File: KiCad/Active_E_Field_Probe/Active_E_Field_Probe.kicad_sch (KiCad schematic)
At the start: 11 parts

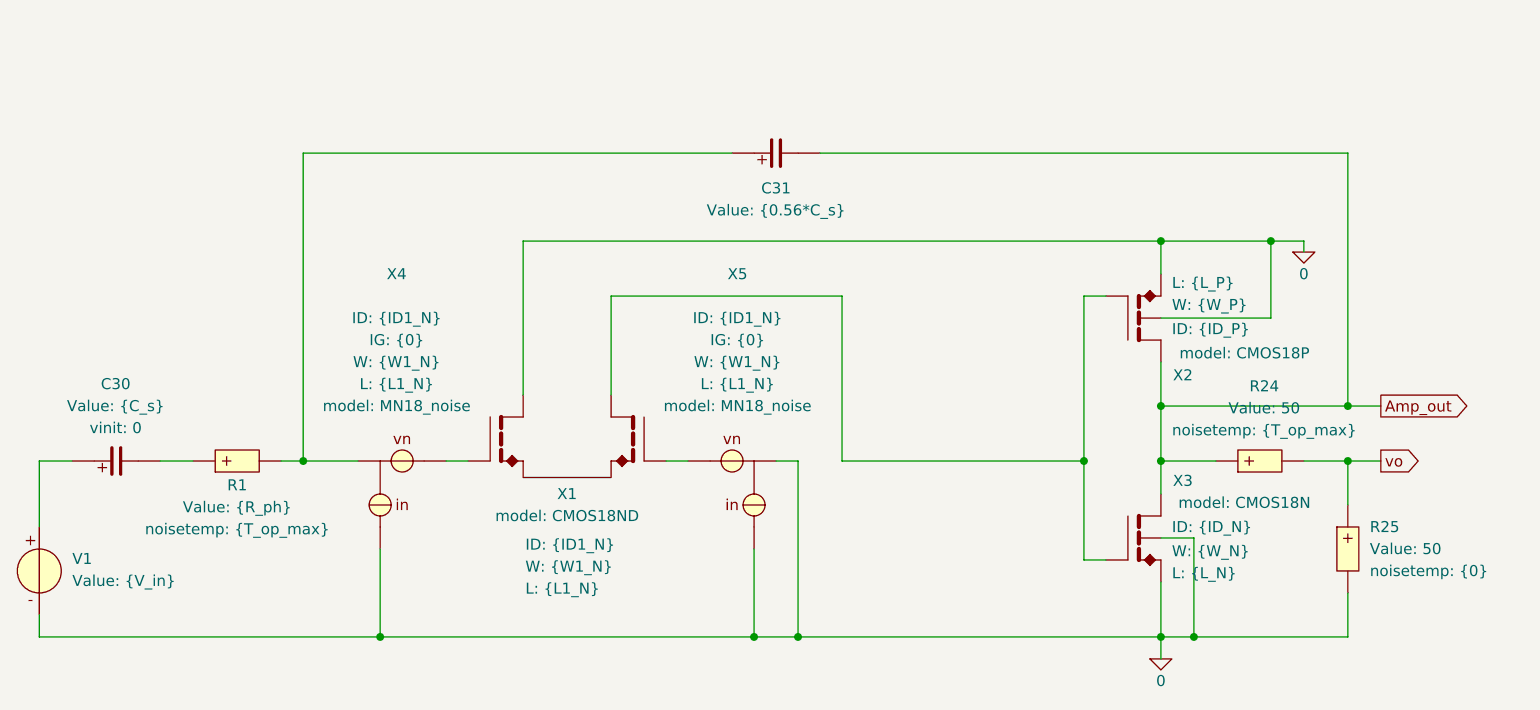
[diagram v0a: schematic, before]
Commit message: cascode
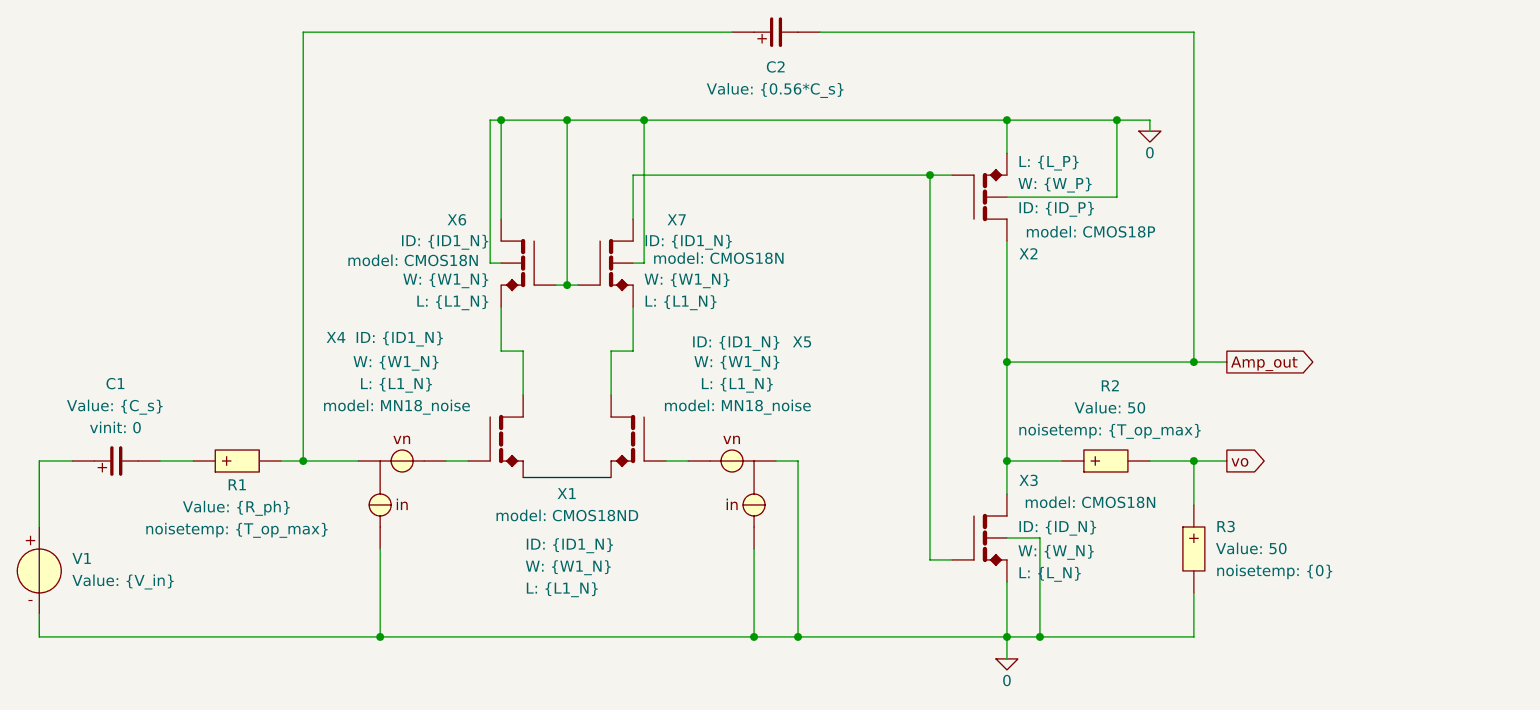
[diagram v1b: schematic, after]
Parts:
- added X6, X7: ~, symbol SLiCAP:XM
- renumbered C30 to C1, C31 to C2, R24 to R2, R25 to R3
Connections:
- net 0: now also X6.1 (D), X6.2 (G), X6.4 (B), X7.2 (G), X7.4 (B); no longer X1.1 (D1)
- net at X2.2 (G), X3.2 (G): now also X7.1 (D); no longer X1.2 (D2)
- new net: X1.2 (D2), X7.3 (S)
- new net: X1.1 (D1), X6.3 (S)
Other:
- moved on the sheet: C2, R2, R3, X2, X3
